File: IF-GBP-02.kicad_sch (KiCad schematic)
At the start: 82 parts, among them CN1 Print Motor, CN2 GB Printer Print Head, CN3 Gameboy Link Port, IC1 4A 8D1, IC2 TMP87CM40AF, IC3 LH5164, IC5 TD62593A, IC6 TD62593A, IC7 458F, J2 Battery Connectors, Q1 B1326, Q10 BR - BCW60DR, Q11 BR - BCW60DR, Q14 24 - DTC114ECA, Q2 FR - 2SA1037, Q3 BR - BCW60DR, Q4 FR, Q5 24 - DTC114ECA, Q6 BF RD, Q7 CF RD, Q8 BR, Q9 FR, SW1 SW_MEC_5E, SW2 SW_DPDT_x2, X1 8 MHz

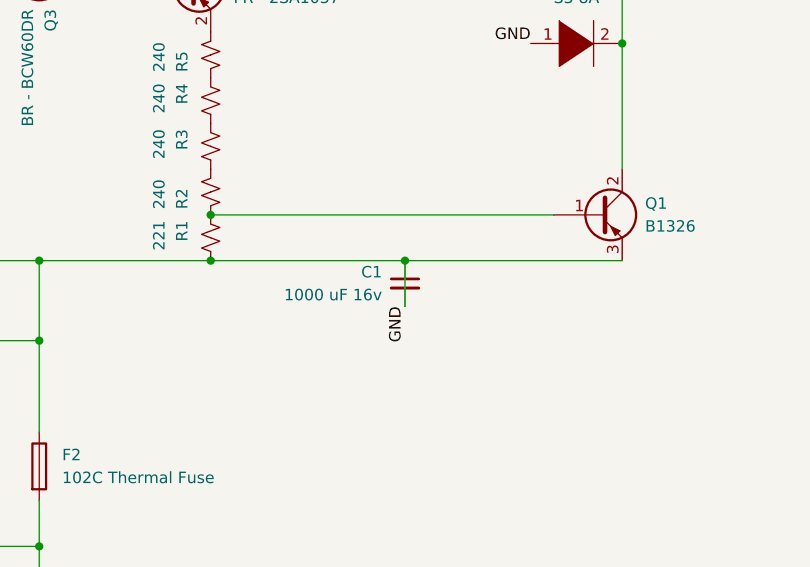
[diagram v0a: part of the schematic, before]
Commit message: Add files via upload
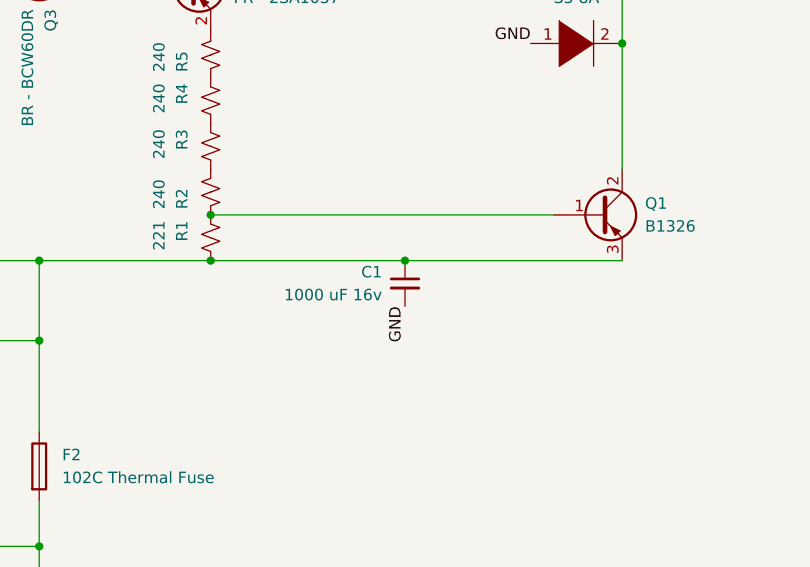
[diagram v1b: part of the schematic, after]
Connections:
- net GND: no longer C1.1, F2.1, Q1.3 (E), R1.1, R16.2, R17.2, R21.1
- new net: C1.1, F2.1, Q1.3 (E), R1.1, R16.2, R17.2, R21.1
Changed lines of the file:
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@@
-    (stroke (width 0) (type default) (color 0 0 0 0))
-  )
-  (wire (pts (xy 477.52 325.12) (xy 477.52 320.04))
     (stroke (width 0) (type default) (color 0 0 0 0))
   )
